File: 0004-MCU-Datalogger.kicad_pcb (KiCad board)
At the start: 2 copper layers, 52.2 x 35.1 mm, 30 parts, among them J1 Conn_01x04_Pin, J2 Conn_01x04_Pin, J3 Conn_01x09_Pin, J4 Conn_02x03_Odd_Even, U1 24LC1025, U2 24LC1025, U3 DS1337S_, U4 ATMEGA328P-AU, Y1 16 MHz, Y2 32.768 KHz

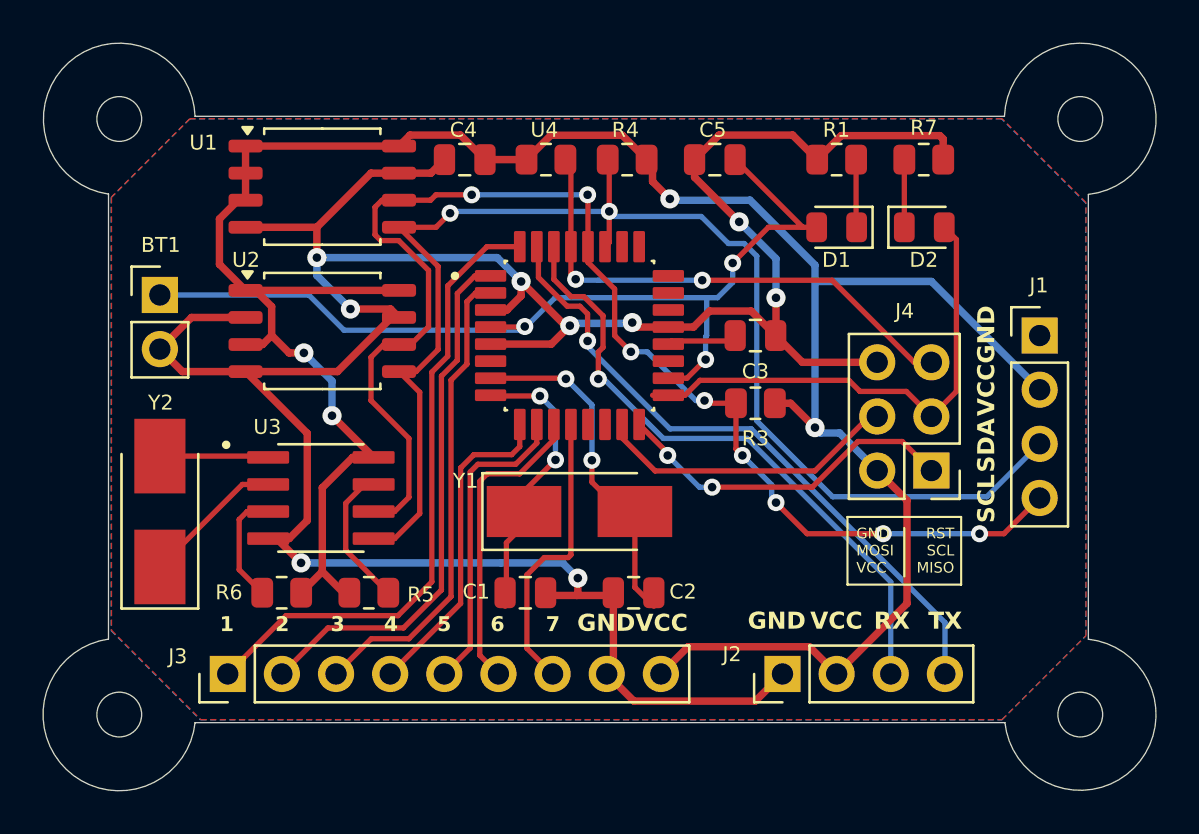
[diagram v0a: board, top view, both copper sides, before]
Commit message: Finalize 4-layer PCB routing
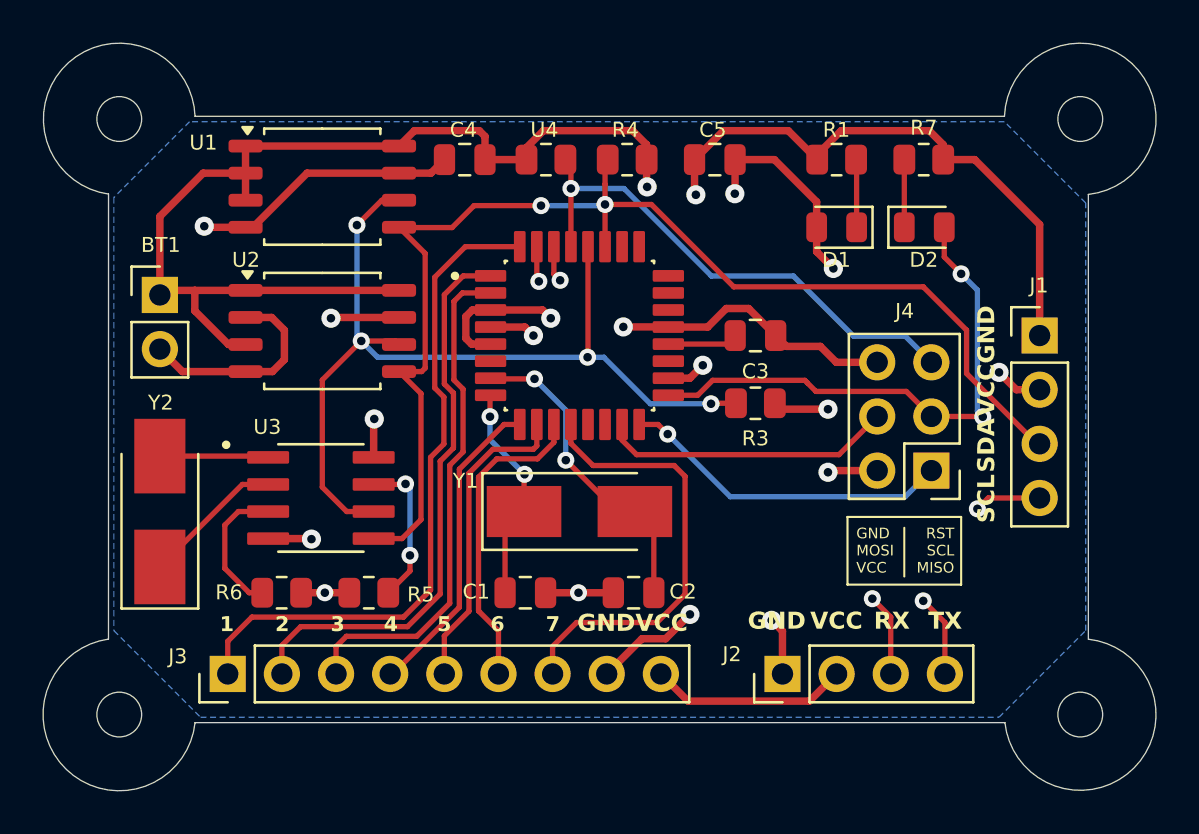
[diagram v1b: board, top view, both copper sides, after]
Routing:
- net /Vcc: track 160.5 -> 84.3 mm, vias 7 -> 10
- net GND: track 138.1 -> 86.2 mm
- net /D8: track 13.7 -> 20.9 mm
- net /SDA: track 64.1 -> 58.9 mm
- net Net-(U4-PB7): track 13.5 -> 10.3 mm
- net /RX: track 29.6 -> 26.7 mm, vias 1 -> 2
- net /D2: track 29.7 -> 31.7 mm
- net /SCK: track 23.7 -> 25.4 mm, vias 0 -> 2
- net /D4: track 22.3 -> 23.9 mm
- net /D3: track 25.2 -> 26.8 mm
- net Net-(U3-~{INTA}): track 5.40 -> 6.55 mm
- net Net-(U4-PB6): track 15.9 -> 14.9 mm
- net /SCL: track 63.1 -> 62.2 mm, vias 8 -> 5
- net /MISO: track 16.4 -> 15.6 mm, vias 2 -> 1
- net /TX: track 30.4 -> 29.8 mm, vias 1 -> 2
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- added copper zone on In2.Cu, net /Vcc
- removed copper zone on F.Cu, net /Vcc
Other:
- copper layers 2 -> 4
